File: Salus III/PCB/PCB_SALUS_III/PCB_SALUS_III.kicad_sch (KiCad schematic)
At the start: 47 parts, among them J1 Conn_01x20_Pin, J2 Conn_01x20_Pin, K1 Relay_SPDT, U1 ESP32-DEVKITC-32D

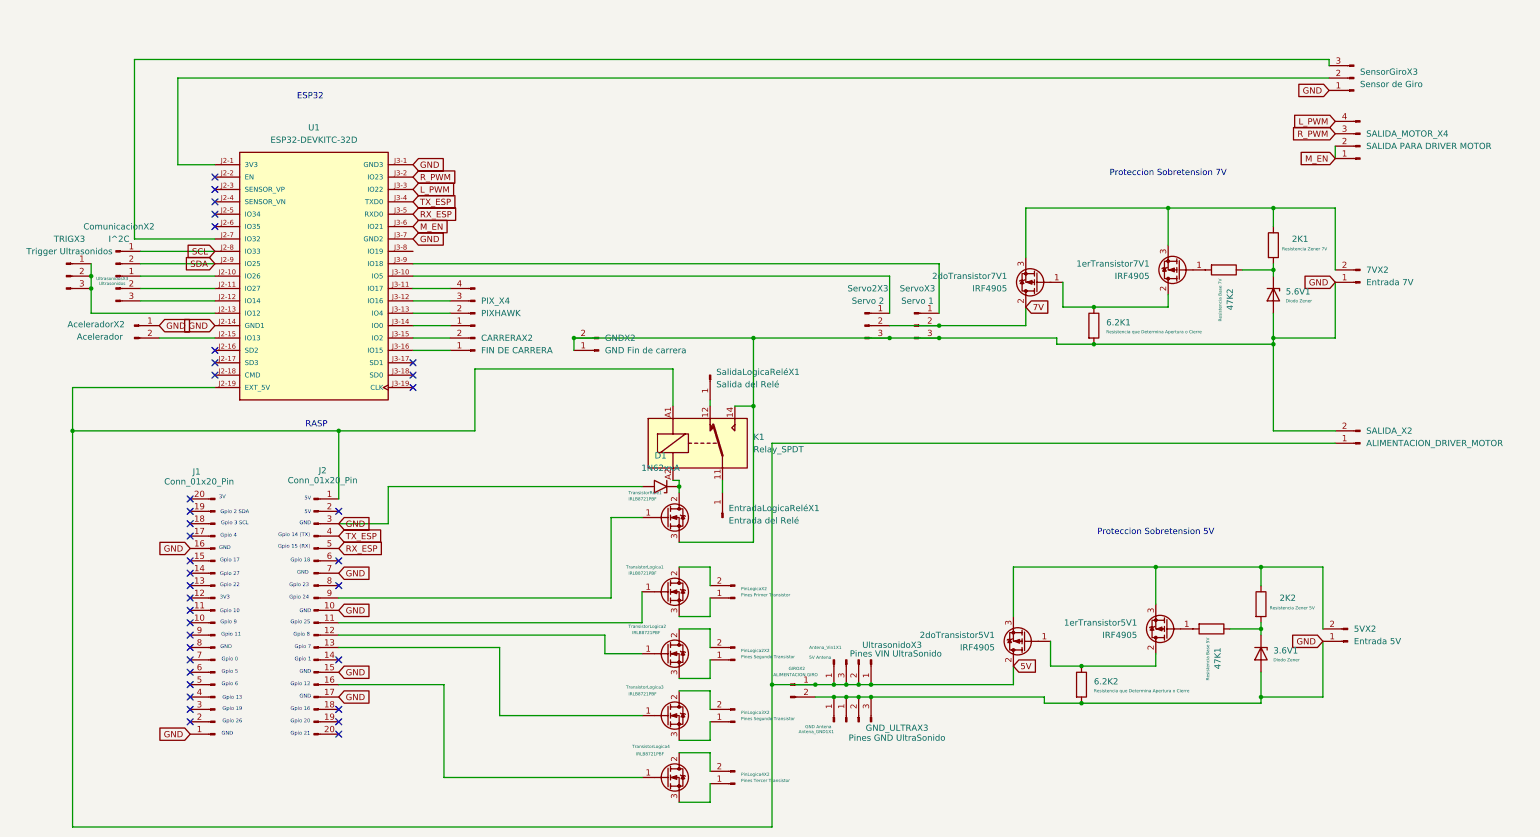
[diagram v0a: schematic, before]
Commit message: Mandar a China
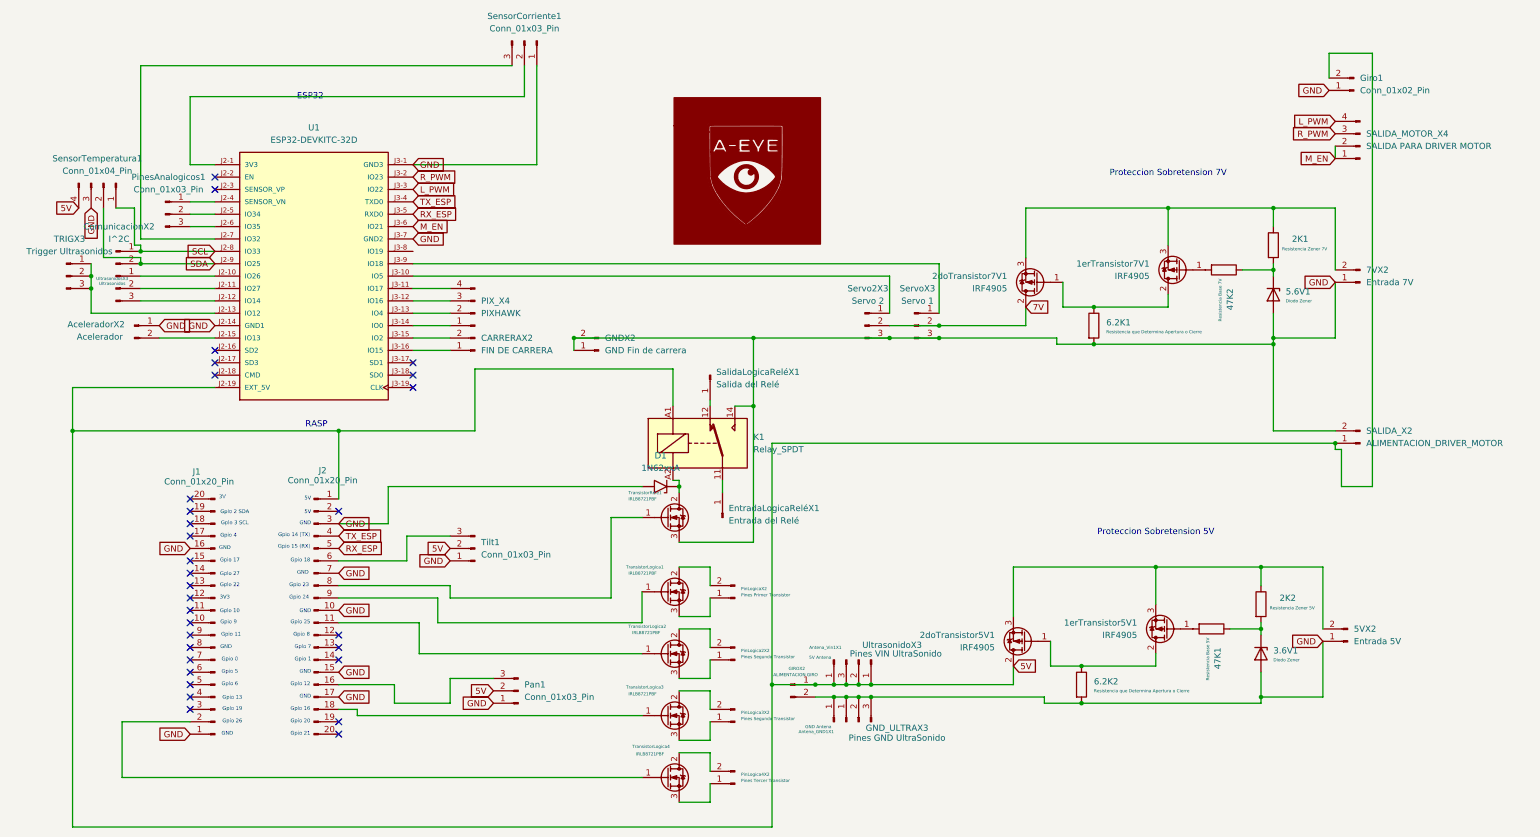
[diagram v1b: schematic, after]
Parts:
- removed SensorGiroX3: Sensor de Giro, Connector_PinHeader_2.54mm:PinHeader_1x03_P2.54mm_Vertical, symbol Connector:Conn_01x03_Pin
- added Giro1: Conn_01x02_Pin, Connector_PinHeader_2.54mm:PinHeader_1x02_P2.54mm_Vertical, symbol Connector:Conn_01x02_Pin
- added Pan1, PinesAnalogicos1, SensorCorriente1, Tilt1: Conn_01x03_Pin, Connector_PinHeader_2.54mm:PinHeader_1x03_P2.54mm_Vertical, symbol Connector:Conn_01x03_Pin
- added SensorTemperatura1: Conn_01x04_Pin, Connector_PinHeader_2.54mm:PinHeader_1x04_P2.54mm_Vertical, symbol Connector:Conn_01x04_Pin
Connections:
- net 5V: now also Giro1.2 (Pin_2), Pan1.2 (Pin_2), SensorTemperatura1.4 (Pin_4), Tilt1.2 (Pin_2)
- net GND: now also Giro1.1 (Pin_1), Pan1.1 (Pin_1), SensorCorriente1.1 (Pin_1), SensorTemperatura1.3 (Pin_3), Tilt1.1 (Pin_1)
- net SCL: now also SensorTemperatura1.1 (Pin_1)
- net SDA: now also SensorTemperatura1.2 (Pin_2)
- net at TransistorLogica1.1 (G): now also J2.9 (Pin_9); no longer J2.11 (Pin_11)
- net at U1.J2-1 (3V3): now also SensorCorriente1.2 (Pin_2)
- net at U1.J2-4 (SENSOR_VN): now also PinesAnalogicos1.1 (Pin_1)
- net at U1.J2-5 (IO34): now also PinesAnalogicos1.2 (Pin_2)
- net at U1.J2-6 (IO35): now also PinesAnalogicos1.3 (Pin_3)
- net at U1.J2-7 (IO32): now also SensorCorriente1.3 (Pin_3)
- net at TransistorLogica4.1 (G): now also J1.2 (Pin_2); no longer J2.16 (Pin_16)
- net at TransistorLogica2.1 (G): now also J2.11 (Pin_11); no longer J2.12 (Pin_12)
- net at TransistorLogica3.1 (G): now also J2.18 (Pin_18); no longer J2.13 (Pin_13)
- net at TransistorRele1.1 (G): now also J2.8 (Pin_8); no longer J2.9 (Pin_9)
- net at J2.6 (Pin_6): now also Tilt1.3 (Pin_3)
- new net: J2.16 (Pin_16), Pan1.3 (Pin_3)
- no-connect marks 36 -> 31
